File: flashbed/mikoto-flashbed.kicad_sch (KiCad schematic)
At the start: 49 parts, among them J1 Conn_01x01, J2 Conn_01x01, J3 Conn_01x01, J4 Conn_01x01, J5 Conn_01x01, J6 Conn_01x01, J7 Conn_01x05, SW1 TVBP06, U1 ProMicro_2

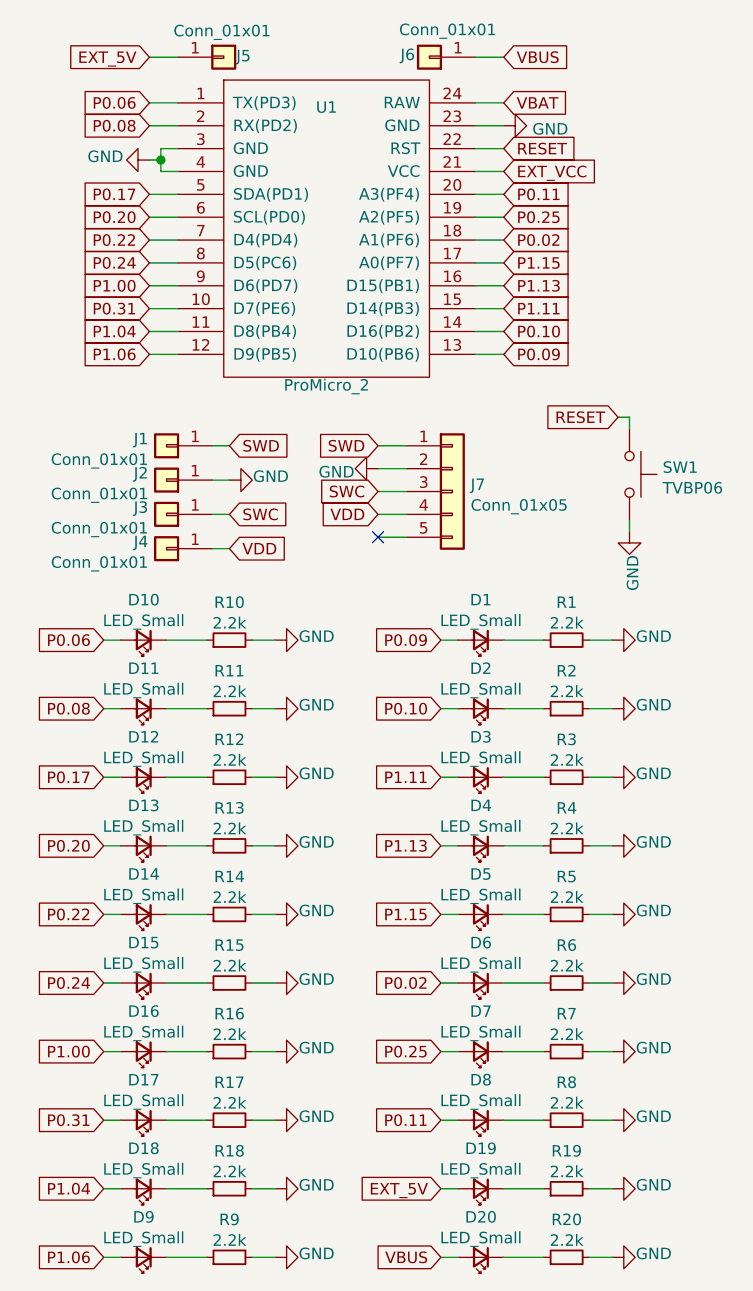
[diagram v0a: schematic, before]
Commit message: update flashbed and add gerbers
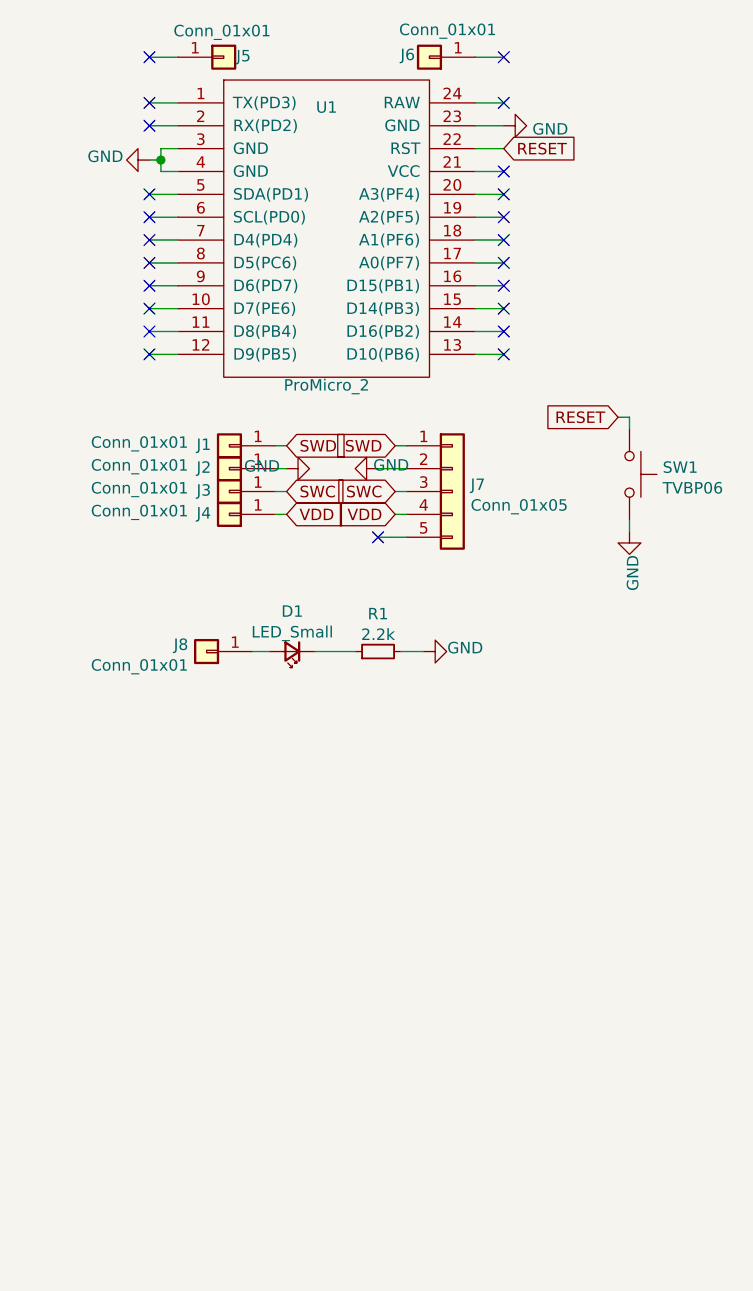
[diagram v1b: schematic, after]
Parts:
- removed D10, D11, D12, D13, D14, D15, D16, D17, D18, D19, D2, D20, D3, D4, D5, D6, D7, D8, D9: LED_Small, LED_SMD:LED_1206_3216Metric_Pad1.42x1.75mm_HandSolder, symbol Device:LED_Small
- removed R10, R11, R12, R13, R14, R15, R16, R17, R18, R19, R2, R20, R3, R4, R5, R6, R7, R8, R9: 2.2k, Resistor_SMD:R_0805_2012Metric_Pad1.15x1.40mm_HandSolder, symbol Device:R_Small
- added J8: Conn_01x01, Connector_PinHeader_2.54mm:PinHeader_1x01_P2.54mm_Vertical, symbol Connector_Generic:Conn_01x01
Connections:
- net EXT_5V: no longer names the net of J5.1 (Pin_1)
- net EXT_VCC: no longer names the net of U1.21 (VCC)
- net P0.02: no longer names the net of U1.18 (A1(PF6))
- net P0.06: no longer names the net of U1.1 (TX(PD3))
- net P0.08: no longer names the net of U1.2 (RX(PD2))
- net P0.09: no longer names the net of D1.2 (A)
- net P0.09: now also J8.1 (Pin_1); no longer U1.13 (D10(PB6))
- net P0.10: no longer names the net of U1.14 (D16(PB2))
- net P0.11: no longer names the net of U1.20 (A3(PF4))
- net P0.17: no longer names the net of U1.5 (SDA(PD1))
- net P0.20: no longer names the net of U1.6 (SCL(PD0))
- net P0.22: no longer names the net of U1.7 (D4(PD4))
- net P0.24: no longer names the net of U1.8 (D5(PC6))
- net P0.25: no longer names the net of U1.19 (A2(PF5))
- net P0.31: no longer names the net of U1.10 (D7(PE6))
- net P1.00: no longer names the net of U1.9 (D6(PD7))
- net P1.04: no longer names the net of U1.11 (D8(PB4))
- net P1.06: no longer names the net of U1.12 (D9(PB5))
- net P1.11: no longer names the net of U1.15 (D14(PB3))
- net P1.13: no longer names the net of U1.16 (D15(PB1))
- net P1.15: no longer names the net of U1.17 (A0(PF7))
- net VBAT: no longer names the net of U1.24 (RAW)
- net VBUS: no longer names the net of J6.1 (Pin_1)
- no-connect marks 1 -> 23
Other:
- moved on the sheet: D1, J1, J2, J3, J4, R1
